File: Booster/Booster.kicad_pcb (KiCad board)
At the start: 2 copper layers, 97 x 60 mm, 124 parts, among them IC401 SN754410, J101 Track, J301 15VDC, J601 StatusLED, J701 Conn_01x04, P201 CONN_01X02, P202 CONN_01X02, P601 ~OVERCURRENT_OUT, P602 ~OVERCURRENT_OUT_OP, P603 MSTR_SW, P604 MSTR_SW_OUT, P605 MSTR_SW_OUT_OP, P606 ~DRIVER_ENABLE_OUT_OP, P607 ~DRIVER_ENABLE_OUT, P701 REVERSER_OUT, P702 REVERSER_OUT_OP, Q601 BC807-40, Q602 BC807-40, Q603 BC807-40, Q604 BC817-40, Q701 BC817-40, SW601 DIP, U201 6N137, U203 LM339, U301 LM7805_TO220, U501 LM338, U502 LM358, U503 NE555, U504 74HC08, U602 PC817, U603 PC817, U604 PC817, U701 74HC86, U702 PC817

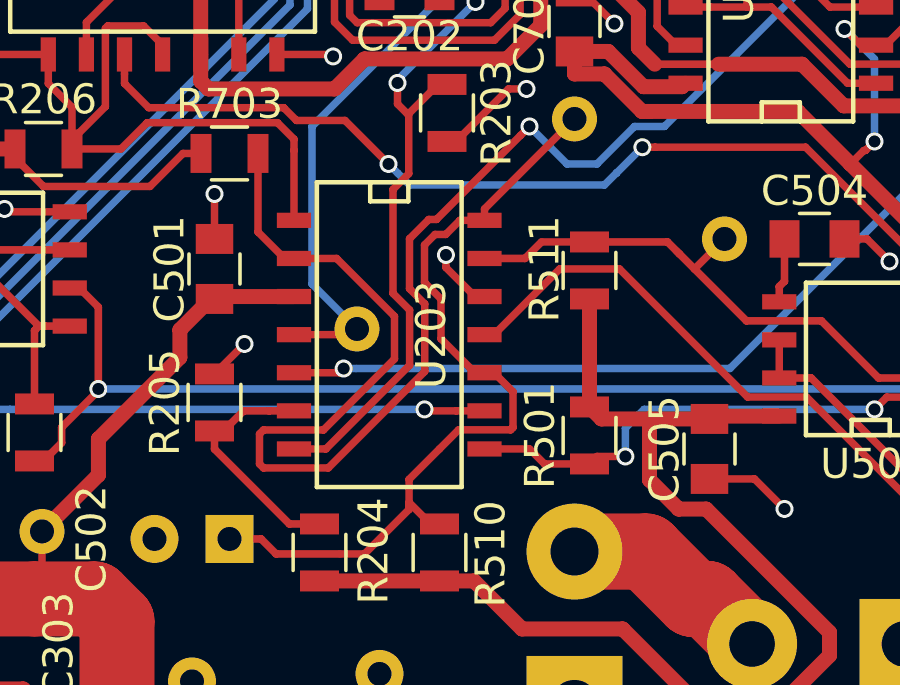
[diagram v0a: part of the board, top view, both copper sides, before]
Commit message: Minor adjustment
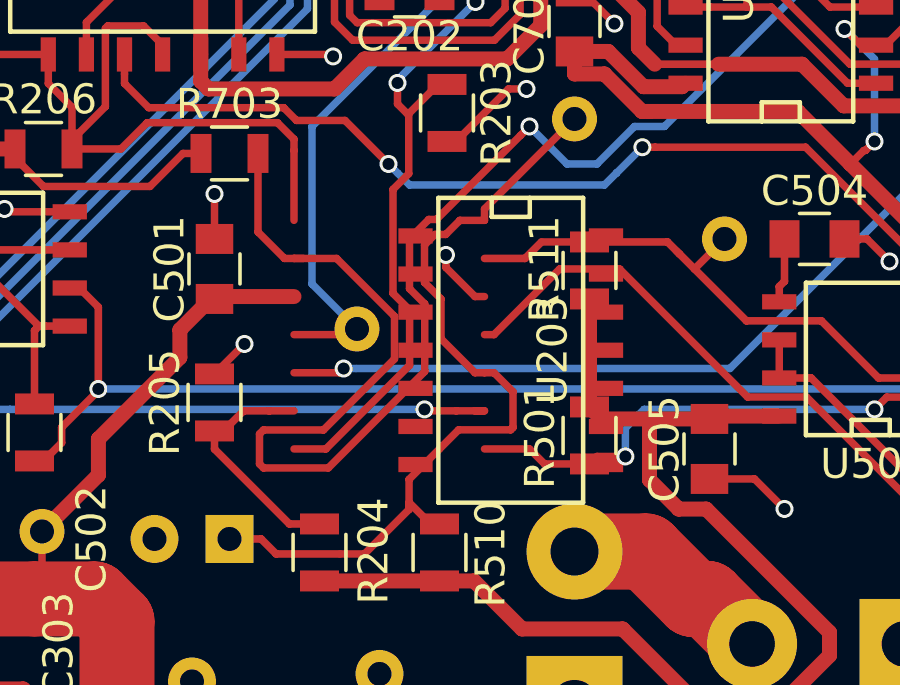
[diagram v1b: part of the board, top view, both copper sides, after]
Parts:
- moved U203 4.08 mm to (161.0, 122.7)
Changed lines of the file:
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@@
   )
   (module SMD_Packages:SOIC-14_N (layer F.Cu)
-    (at 156.952 122.19 270)
+    (at 161.002 122.71 270)
     (descr "Module CMS SOJ 14 pins Large")
     (tags "CMS SOJ")

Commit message: Turns out last minor adjustment was actually an error. :)
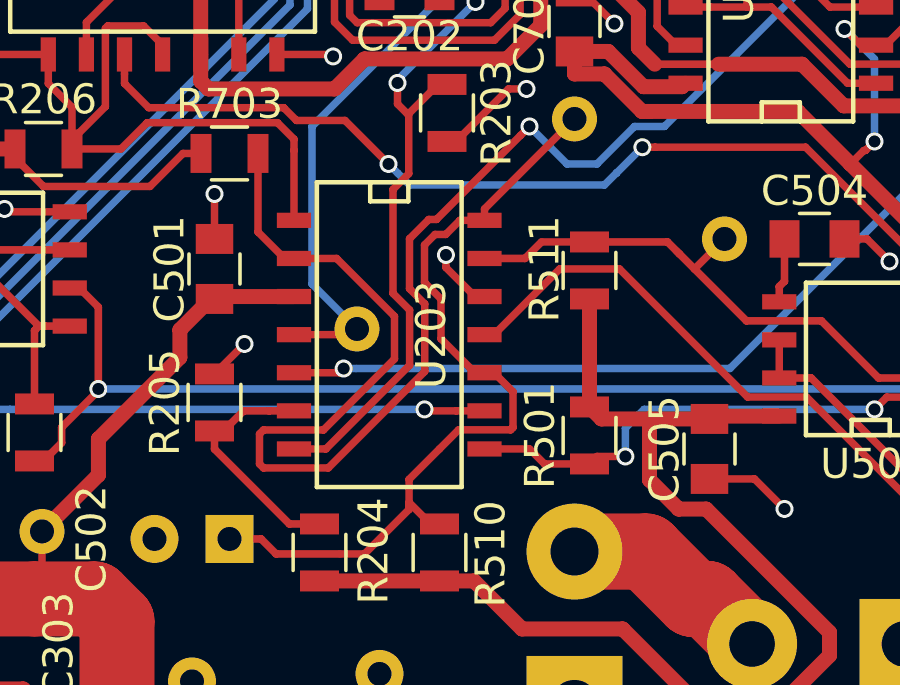
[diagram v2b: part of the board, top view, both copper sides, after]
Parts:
- moved U203 4.08 mm to (157.0, 122.2)
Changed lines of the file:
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@@
   )
   (module SMD_Packages:SOIC-14_N (layer F.Cu)
-    (at 161.002 122.71 270)
+    (at 156.952 122.19 270)
     (descr "Module CMS SOJ 14 pins Large")
     (tags "CMS SOJ")
